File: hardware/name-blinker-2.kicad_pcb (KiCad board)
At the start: 2 copper layers, 70 x 50 mm, 40 parts, among them M1 MOUNTING-HOLE, M10 MOUNTING-HOLE, M12 MOUNTING-HOLE, M13 MOUNTING-HOLE, M2 MOUNTING-HOLE, M3 MOUNTING-HOLE, M4 MOUNTING-HOLE, M5 MOUNTING-HOLE, M6 MOUNTING-HOLE, M7 MOUNTING-HOLE, M8 MOUNTING-HOLE, M9 MOUNTING-HOLE, P1 CONN_01X08, P2 USB_OTG, SW2 SMD-TOGGLE-SWITCH-2CH_2X3P-7X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, U1 MCP73831, U2 BMD-300, U3 TPS63051

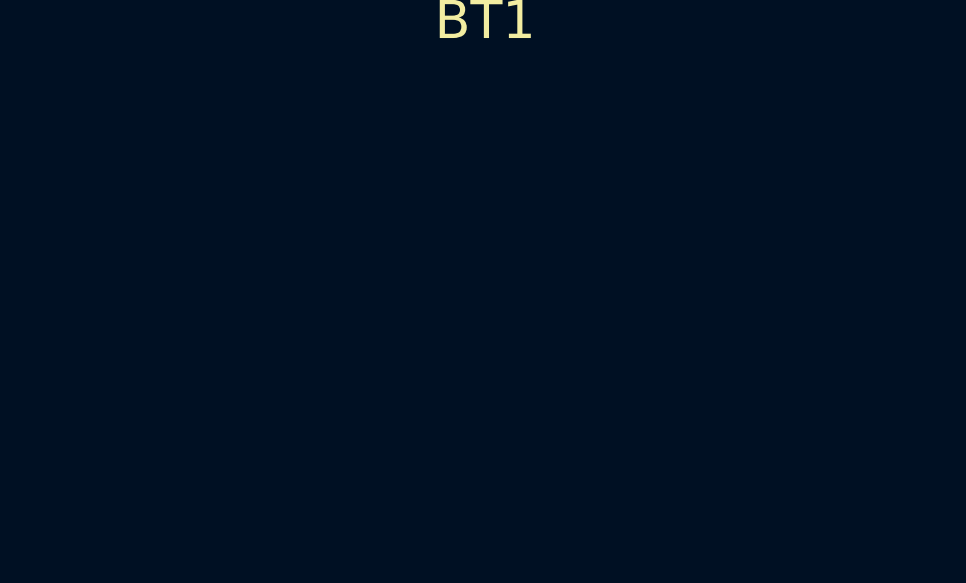
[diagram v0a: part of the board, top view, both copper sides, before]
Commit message: add inductor
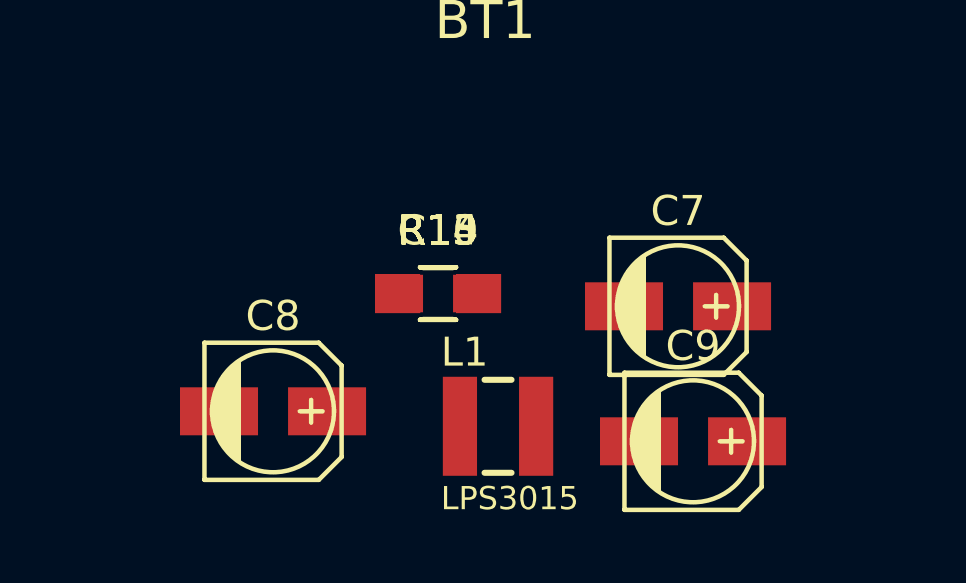
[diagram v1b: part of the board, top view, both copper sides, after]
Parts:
- added C10: 1nF, Capacitors_SMD:C_0805_HandSoldering, F.Cu at (185.0, 105.1)
- added C7: 10uF, Capacitors_SMD:c_elec_4x5.8, F.Cu at (193.0, 105.5)
- added C8: 10uF, Capacitors_SMD:c_elec_4x5.8, F.Cu at (179.5, 109.0)
- added C9: 10uF, Capacitors_SMD:c_elec_4x5.8, F.Cu at (193.5, 110.0)
- added L1: LPS3015, lps3015:LPS3015, F.Cu at (187.0, 109.5)
- added R13: 1M, Resistors_SMD:R_0805_HandSoldering, F.Cu at (185.0, 105.1)
- added R14: 800K, Resistors_SMD:R_0805_HandSoldering, F.Cu at (185.0, 105.1)
- added R15: 2M, Resistors_SMD:R_0805_HandSoldering, F.Cu at (185.0, 105.1)
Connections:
- C3 pad 2: GND -> Net-(C3-Pad2)
- C6 pad 1: VCC -> +3V3
- M12 pad 1: VCC -> +3V3
- P1 pad 2: VCC -> +3V3
- P1 pad 4: GND -> UART_TX
- P1 pad 5: SWDIO -> UART_RX
- P1 pad 6: SWCLK -> SWDIO
- P1 pad 7: UART_TX -> SWCLK
- P1 pad 8: UART_RX -> GND
- U2 pad P17: VCC -> +3V3
- U3 pad P$10: Net-(U3-PadP$10) -> VCC
- U3 pad P$11: Net-(U3-PadP$11) -> VCC
- U3 pad P$12: Net-(U3-PadP$12) -> VCC
- U3 pad P$2: Net-(U3-PadP$2) -> GND
- U3 pad P$4: Net-(U3-PadP$4) -> +3V3
- U3 pad P$5: Net-(U3-PadP$5) -> +3V3
- U3 pad P$6: Net-(U3-PadP$6) -> GND
- U3 pad P$9: Net-(U3-PadP$9) -> GND
